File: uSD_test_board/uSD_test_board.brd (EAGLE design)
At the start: 22.9 x 99.1 mm, 6 parts

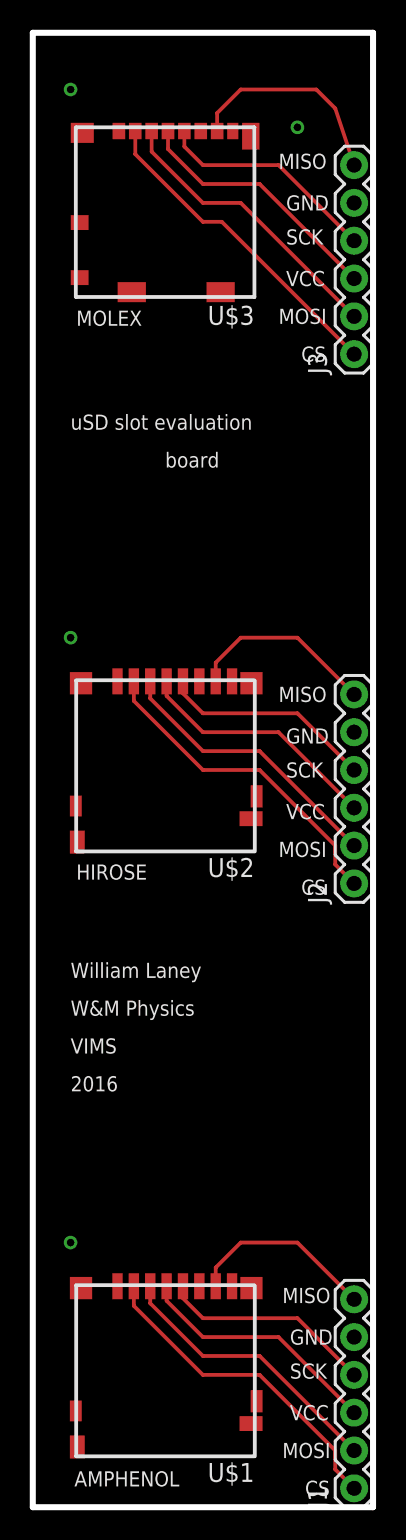
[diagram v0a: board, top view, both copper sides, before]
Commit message: prep for fab
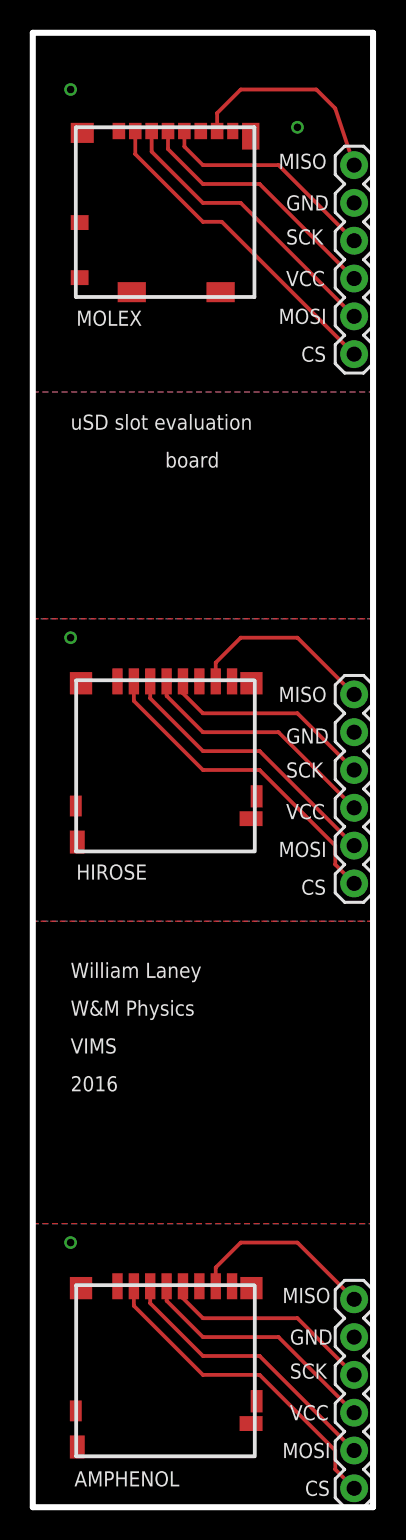
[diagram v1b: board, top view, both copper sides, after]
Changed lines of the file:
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@@
 <setting verticaltext="up"/>
 </settings>
-<grid distance="0.05" unitdist="inch" unit="inch" style="lines" multiple="1" display="yes" altdistance="0.025" altunitdist="inch" altunit="inch"/>
+<grid distance="0.05" unitdist="inch" unit="inch" style="lines" multiple="1" display="yes" altdistance="0.005" altunitdist="inch" altunit="inch"/>
 <layers>
 <layer number="1" name="Top" color="4" fill="1" visible="yes" active="yes"/>
@@
 </class>
 </classes>
-<designrules name="default">
+<designrules name="oshpark-2layer">
 <description language="de">&lt;b&gt;EAGLE Design Rules&lt;/b&gt;
 &lt;p&gt;
@@
 Einstellungen hier und speichern die Design Rules unter
 einem neuen Namen ab.</description>
-<description language="en">&lt;b&gt;EAGLE Design Rules&lt;/b&gt;
+<description language="en">&lt;b&gt;Laen's PCB Order Design Rules&lt;/b&gt;
 &lt;p&gt;
-The default Design Rules have been set to cover
-a wide range of applications. Your particular design
-may have different requirements, so please make the
-necessary adjustments and save your customized
-design rules under a new name.</description>
+Please make sure your boards conform to these design rules.</description>
 <param name="layerSetup" value="(1*16)"/>
-<param name="mtCopper" value="0.035mm 0.035mm 0.035mm 0.035mm 0.035mm 0.035mm 0.035mm 0.035mm 0.035mm 0.035mm 0.035mm 0.035mm 0.035mm 0.035mm 0.035mm 0.035mm"/>
-<param name="mtIsolate" value="1.5mm 0.15mm 0.2mm 0.15mm 0.2mm 0.15mm 0.2mm 0.15mm 0.2mm 0.15mm 0.2mm 0.15mm 0.2mm 0.15mm 0.2mm"/>
-<param name="mdWireWire" value="8mil"/>
-<param name="mdWirePad" value="8mil"/>
-<param name="mdWireVia" value="8mil"/>
-<param name="mdPadPad" value="8mil"/>
-<param name="mdPadVia" value="8mil"/>
-<param name="mdViaVia" value="8mil"/>
-<param name="mdSmdPad" value="8mil"/>
-<param name="mdSmdVia" value="8mil"/>
-<param name="mdSmdSmd" value="8mil"/>
+<param name="mtCopper" value="0.0356mm 0.0356mm 0.0356mm 0.0356mm 0.0356mm 0.0356mm 0.0356mm 0.0356mm 0.0356mm 0.0356mm 0.0356mm 0.0356mm 0.0356mm 0.0356mm 0.0356mm 0.0356mm"/>
+<param name="mtIsolate" value="1.5011mm 0.1499mm 0.2007mm 0.1499mm 0.2007mm 0.1499mm 0.2007mm 0.1499mm 0.2007mm 0.1499mm 0.2007mm 0.1499mm 0.2007mm 0.1499mm 0.2007mm"/>
+<param name="mdWireWire" value="6mil"/>
+<param name="mdWirePad" value="6mil"/>
+<param name="mdWireVia" value="6mil"/>
+<param name="mdPadPad" value="6mil"/>
+<param name="mdPadVia" value="6mil"/>
+<param name="mdViaVia" value="6mil"/>
+<param name="mdSmdPad" value="6mil"/>
+<param name="mdSmdVia" value="6mil"/>
+<param name="mdSmdSmd" value="6mil"/>
 <param name="mdViaViaSameLayer" value="8mil"/>
 <param name="mnLayersViaInSmd" value="2"/>
-<param name="mdCopperDimension" value="40mil"/>
-<param name="mdDrill" value="8mil"/>
+<param name="mdCopperDimension" value="15mil"/>
+<param name="mdDrill" value="6mil"/>
 <param name="mdSmdStop" value="0mil"/>
-<param name="msWidth" value="10mil"/>
-<param name="msDrill" value="24mil"/>
-<param name="msMicroVia" value="9.99mm"/>
+<param name="msWidth" value="6mil"/>
+<param name="msDrill" value="13mil"/>
+<param name="msMicroVia" value="13mil"/>
 <param name="msBlindViaRatio" value="0.5"/>
 <param name="rvPadTop" value="0.25"/>
@@
 <param name="rvMicroViaOuter" value="0.25"/>
 <param name="rvMicroViaInner" value="0.25"/>
-<param name="rlMinPadTop" value="10mil"/>
+<param name="rlMinPadTop" value="7mil"/>
 <param name="rlMaxPadTop" value="20mil"/>
-<param name="rlMinPadInner" value="10mil"/>
+<param name="rlMinPadInner" value="7mil"/>
 <param name="rlMaxPadInner" value="20mil"/>
-<param name="rlMinPadBottom" value="10mil"/>
+<param name="rlMinPadBottom" value="7mil"/>
 <param name="rlMaxPadBottom" value="20mil"/>
-<param name="rlMinViaOuter" value="8mil"/>
+<param name="rlMinViaOuter" value="7mil"/>
 <param name="rlMaxViaOuter" value="20mil"/>
-<param name="rlMinViaInner" value="8mil"/>
+<param name="rlMinViaInner" value="7mil"/>
 <param name="rlMaxViaInner" value="20mil"/>
 <param name="rlMinMicroViaOuter" value="4mil"/>
@@
 <param name="mvStopFrame" value="1"/>
 <param name="mvCreamFrame" value="0"/>
-<param name="mlMinStopFrame" value="4mil"/>
-<param name="mlMaxStopFrame" value="4mil"/>
+<param name="mlMinStopFrame" value="2.5mil"/>
+<param name="mlMaxStopFrame" value="2.5mil"/>
 <param name="mlMinCreamFrame" value="0mil"/>
 <param name="mlMaxCreamFrame" value="0mil"/>
@@
 </autorouter>
 <elements>
-<element name="J1" library="SparkFun-Connectors" package="1X06" value="" x="21.59" y="1.27" rot="R90">
+<element name="J1" library="SparkFun-Connectors" package="1X06" value="" x="21.59" y="1.27" smashed="yes" rot="R90">
 <attribute name="PROD_ID" value="CONN-08437" x="21.59" y="1.27" size="1.778" layer="27" rot="R90" display="off"/>
-</element>
-<element name="J2" library="SparkFun-Connectors" package="1X06" value="" x="21.59" y="41.91" rot="R90">
+<attribute name="VALUE" x="24.765" y="0" size="1.27" layer="27" rot="R90"/>
+</element>
+<element name="J2" library="SparkFun-Connectors" package="1X06" value="" x="21.59" y="41.91" smashed="yes" rot="R90">
 <attribute name="PROD_ID" value="CONN-08437" x="21.59" y="41.91" size="1.778" layer="27" rot="R90" display="off"/>
-</element>
-<element name="J3" library="SparkFun-Connectors" package="1X06" value="" x="21.59" y="77.47" rot="R90">
+<attribute name="VALUE" x="24.765" y="40.64" size="1.27" layer="27" rot="R90"/>
+</element>
+<element name="J3" library="SparkFun-Connectors" package="1X06" value="" x="21.59" y="77.47" smashed="yes" rot="R90">
 <attribute name="PROD_ID" value="CONN-08437" x="21.59" y="77.47" size="1.778" layer="27" rot="R90" display="off"/>
-</element>
-<element name="U$1" library="sharkdunio" package="AMPHENOL_MICROSD" value="AMPHENOL_MICROSD" x="8.89" y="13.97" rot="R180"/>
-<element name="U$2" library="sharkdunio" package="AMPHENOL_MICROSD" value="HIROSE_MICROSD" x="8.89" y="54.61" rot="R180"/>
-<element name="U$3" library="sharkdunio" package="MOLEX_MICROSD" value="MOLEX_MICROSD" x="8.89" y="92.71" rot="R180"/>
+<attribute name="VALUE" x="24.765" y="76.2" size="1.27" layer="27" rot="R90"/>
+</element>
+<element name="U$1" library="sharkdunio" package="AMPHENOL_MICROSD" value="AMPHENOL_MICROSD" x="8.89" y="13.97" smashed="yes" rot="R180">
+<attribute name="VALUE" x="14.89" y="17.47" size="1.27" layer="27" rot="R180"/>
+</element>
+<element name="U$2" library="sharkdunio" package="AMPHENOL_MICROSD" value="HIROSE_MICROSD" x="8.89" y="54.61" smashed="yes" rot="R180">
+<attribute name="VALUE" x="14.89" y="58.11" size="1.27" layer="27" rot="R180"/>
+</element>
+<element name="U$3" library="sharkdunio" package="MOLEX_MICROSD" value="MOLEX_MICROSD" x="8.89" y="92.71" smashed="yes" rot="R180">
+<attribute name="VALUE" x="14.89" y="94.71" size="1.27" layer="27" rot="R180"/>
+</element>
 </elements>
 <signals>
@@
 <contactref element="U$3" pad="6"/>
 <contactref element="J3" pad="5"/>
-<polygon width="0.4064" layer="1" isolate="0.3048">
-<vertex x="0" y="0"/>
-<vertex x="22.86" y="0"/>
-<vertex x="22.86" y="1.27"/>
-<vertex x="22.86" y="99.06"/>
-<vertex x="0" y="99.06"/>
-</polygon>
-<polygon width="0.254" layer="16" isolate="0.3048">
-<vertex x="0" y="99.06"/>
-<vertex x="22.86" y="99.06"/>
-<vertex x="22.86" y="0"/>
-<vertex x="0" y="0"/>
-</polygon>
 <via x="17.78" y="92.71" extent="1-16" drill="0.508"/>
 <via x="2.54" y="17.78" extent="1-16" drill="0.508"/>
 <via x="2.54" y="58.42" extent="1-16" drill="0.508"/>
 <via x="2.54" y="95.25" extent="1-16" drill="0.508"/>
+<polygon width="0.254" layer="16" isolate="0.3048">
+<vertex x="0" y="99.06"/>
+<vertex x="0" y="74.93"/>
+<vertex x="22.86" y="74.93"/>
+<vertex x="22.86" y="99.06"/>
+</polygon>
+<polygon width="0.254" layer="1" isolate="0.3048">
+<vertex x="0" y="99.06"/>
+<vertex x="0" y="74.93"/>
+<vertex x="22.86" y="74.93"/>
+<vertex x="22.86" y="99.06"/>
+</polygon>
+<polygon width="0.254" layer="1" isolate="0.3048">
+<vertex x="0" y="59.69"/>
+<vertex x="22.86" y="59.69"/>
+<vertex x="22.86" y="39.37"/>
+<vertex x="0" y="39.37"/>
+</polygon>
+<polygon width="0.254" layer="16" isolate="0.3048">
+<vertex x="0" y="59.69"/>
+<vertex x="0" y="39.37"/>
+<vertex x="22.86" y="39.37"/>
+<vertex x="22.86" y="59.69"/>
+</polygon>
+<polygon width="0.254" layer="16" isolate="0.3048">
+<vertex x="0" y="19.05"/>
+<vertex x="22.86" y="19.05"/>
+<vertex x="22.86" y="0"/>
+<vertex x="0" y="0"/>
+</polygon>
+<polygon width="0.254" layer="1" isolate="0.3048">
+<vertex x="0" y="19.05"/>
+<vertex x="22.86" y="19.05"/>
+<vertex x="22.86" y="0"/>
+<vertex x="0" y="0"/>
+</polygon>
+<wire x1="21.59" y1="52.07" x2="11.19" y2="14.845" width="0" layer="19" extent="1-1"/>
+<wire x1="6.65" y1="81.635" x2="2.54" y2="58.42" width="0" layer="19" extent="1-1"/>
 </signal>
 <signal name="DO1">
